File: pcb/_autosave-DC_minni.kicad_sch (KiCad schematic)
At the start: 54 parts, among them J1 DRUCKSENSOR, J2 Encoder, U1 ESP32-DevKitC, U2 USB-C to DIP PCB

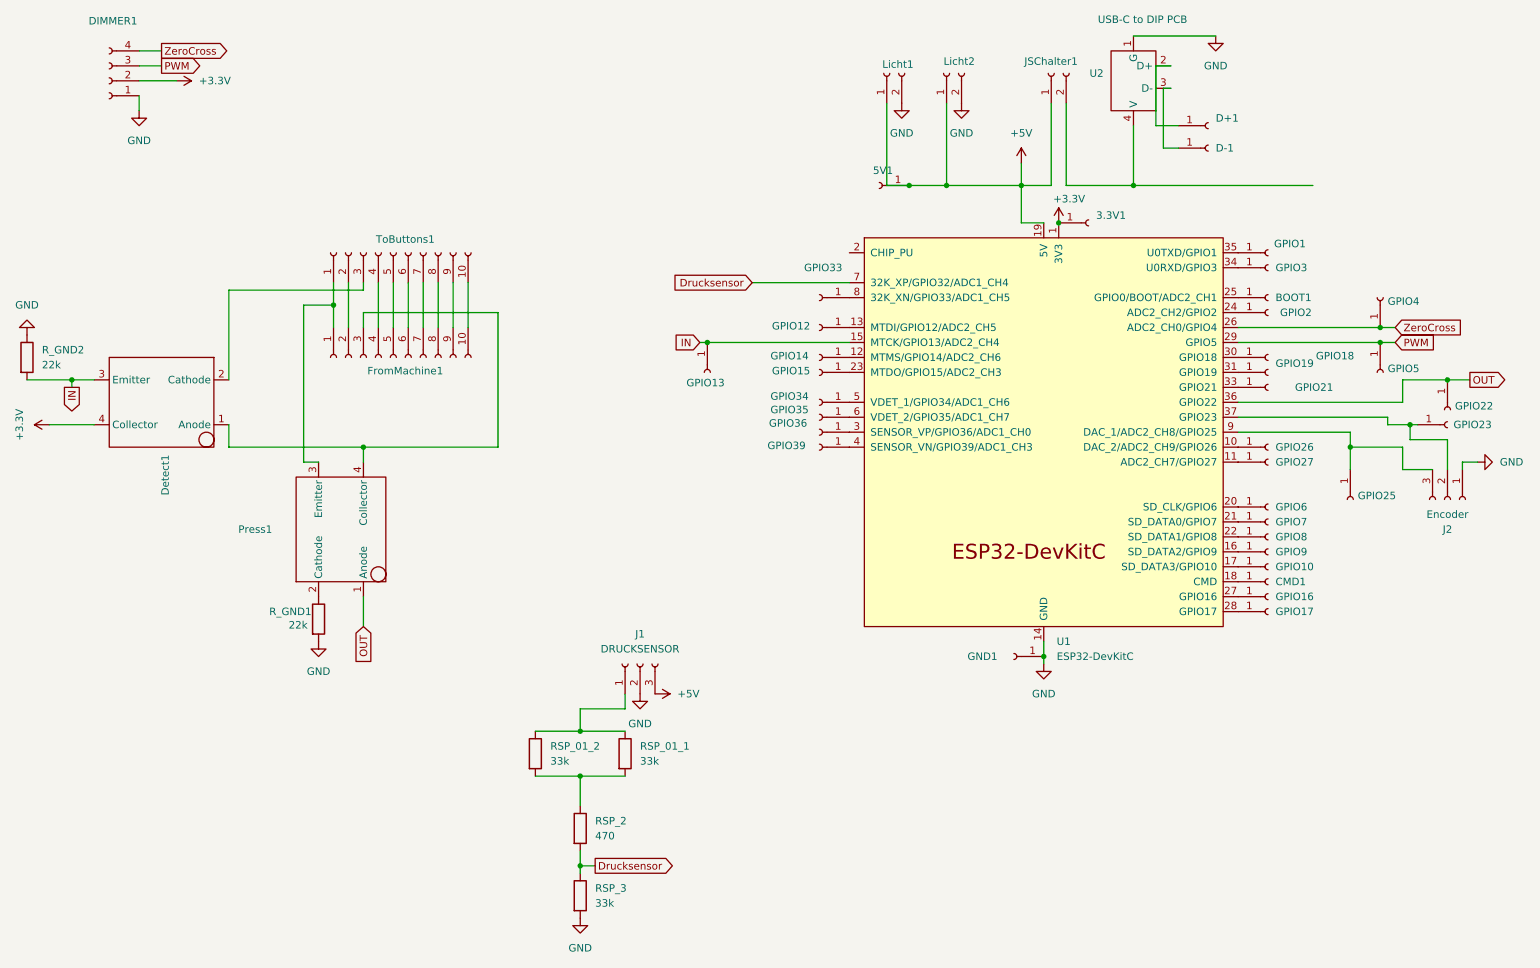
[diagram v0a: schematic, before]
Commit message: Implement comments from Review
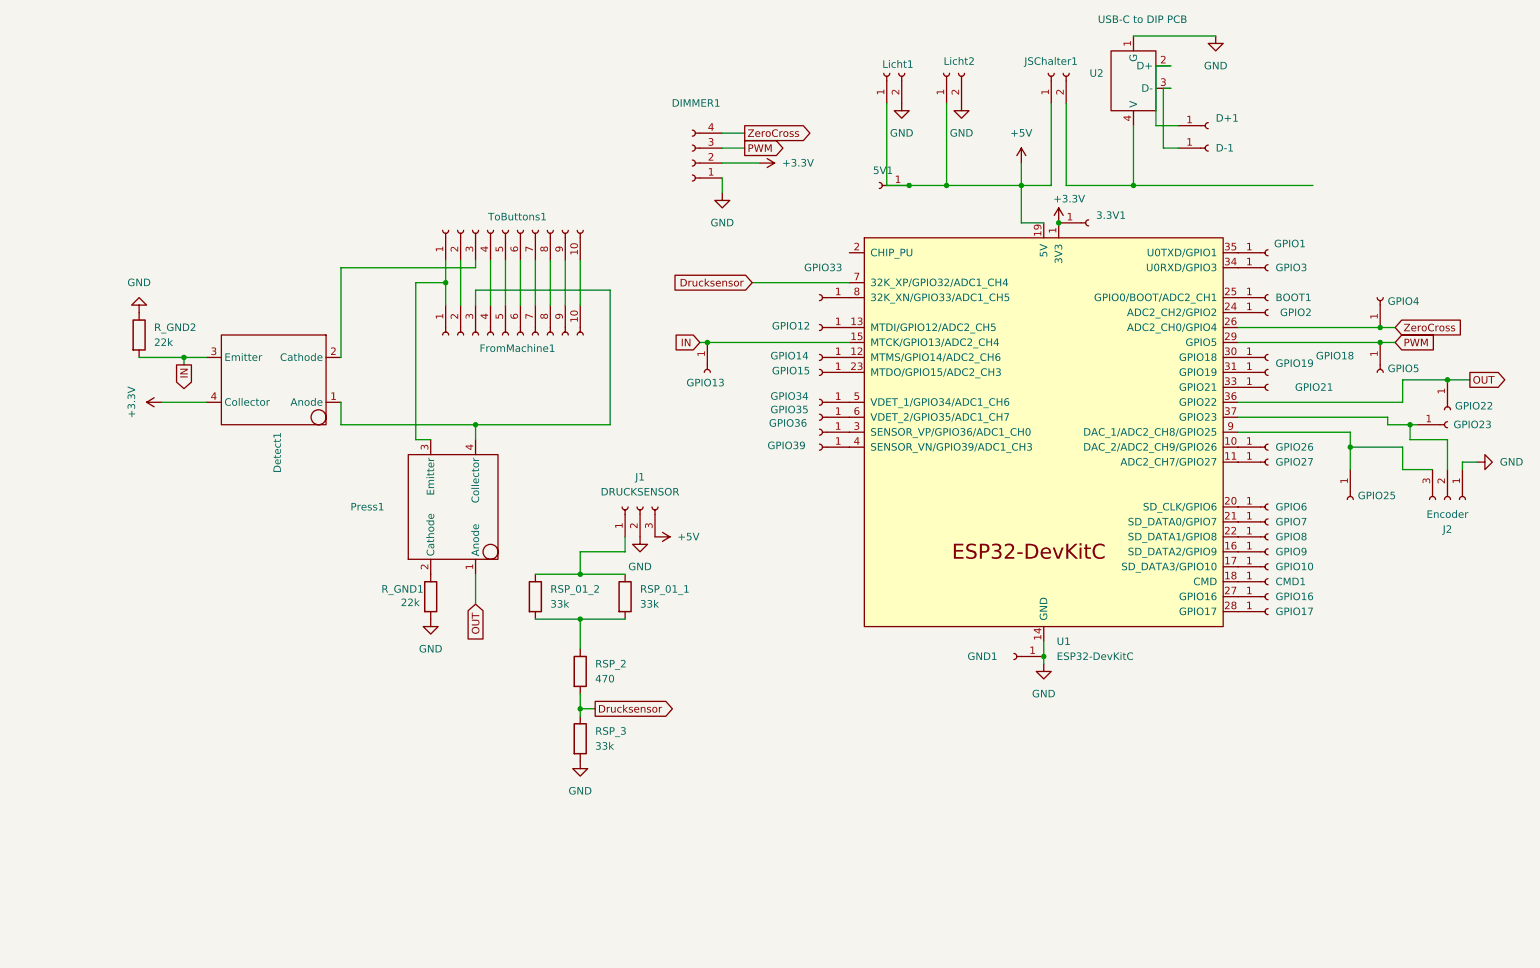
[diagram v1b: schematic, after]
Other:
- moved on the sheet: DIMMER1, Detect1, FromMachine1, J1, Press1, RSP_01_1, RSP_01_2, RSP_2, RSP_3, R_GND1, R_GND2, ToButtons1
